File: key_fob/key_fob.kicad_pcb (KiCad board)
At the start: 2 copper layers, 20 parts, among them IC1 L4931ABDT33-TR, J1 Arduino-NANO-33, J2 B2B-PH-K-S_LF__SN_, U1 PS1240P02BT

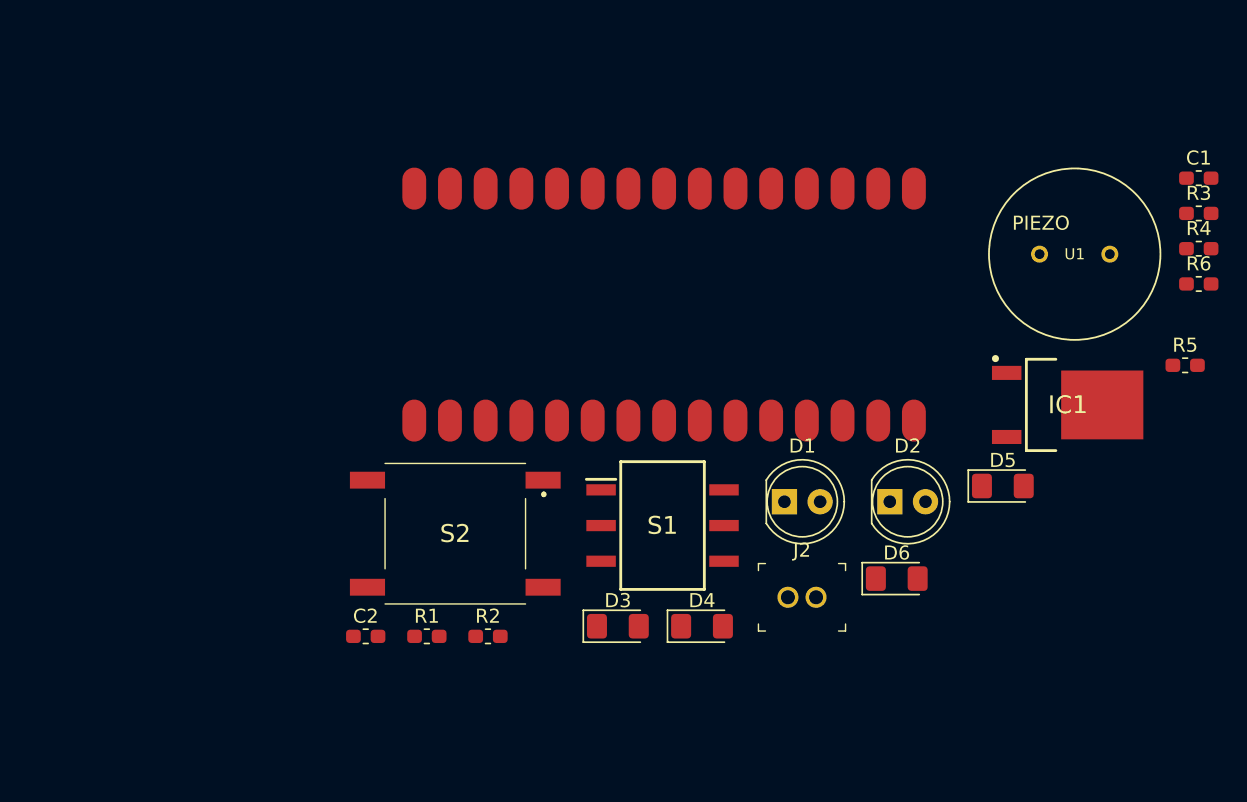
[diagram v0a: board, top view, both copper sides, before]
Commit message: Got some stuff started for key fod pcb
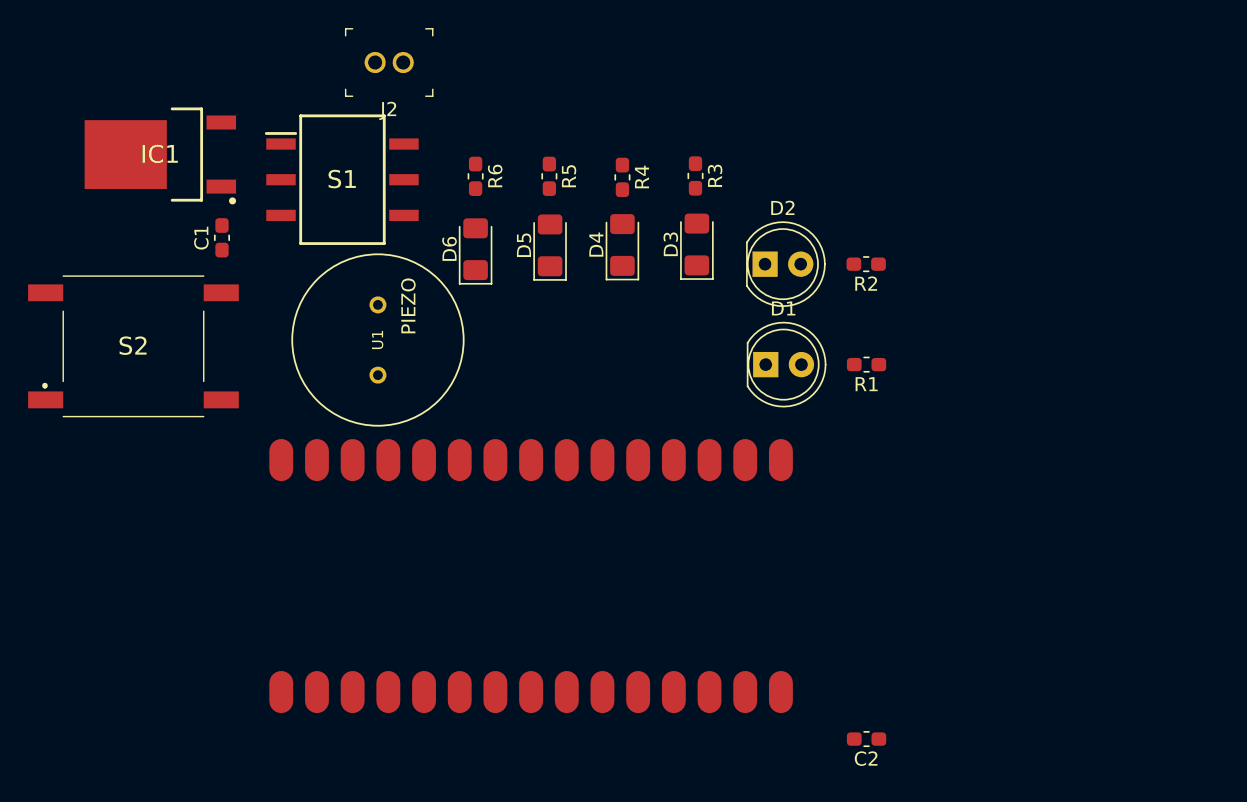
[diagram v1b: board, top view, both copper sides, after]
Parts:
- moved C1 69.6 mm to (20.6, 47.4), turned to 90 degrees
- moved IC1 67.0 mm to (16.2, 41.5), turned to 180 degrees
- moved R6 52.0 mm to (38.7, 43.0), turned to 270 degrees
- moved U1 50.0 mm to (31.8, 54.7), turned to 270 degrees
- moved R5 47.2 mm to (44.0, 43.0), turned to 270 degrees
- moved J2 46.9 mm to (33.5, 35.0), turned to 180 degrees
- moved R4 41.3 mm to (49.1, 43.1), turned to 270 degrees
- moved D6 38.1 mm to (38.7, 48.2), turned to 90 degrees
- moved R2 37.8 mm to (66.5, 49.3), turned to 180 degrees
- moved R1 36.8 mm to (66.5, 56.5), turned to 180 degrees
- moved D5 36.5 mm to (44.0, 48.0), turned to 90 degrees
- moved C2 36.4 mm to (66.5, 83.1), turned to 180 degrees
- moved R3 35.9 mm to (54.4, 43.0), turned to 270 degrees
- moved S1 33.5 mm to (29.2, 43.3)
- moved D3 27.7 mm to (54.5, 47.9), turned to 90 degrees
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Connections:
- S1 pad 1: +BATT -> +3V3
- S1 pad 2: +3V3 -> +BATT
- S1 pad 5: LED_SW -> POWER_SW
- S1 pad 6: POWER_SW -> LED_SW
